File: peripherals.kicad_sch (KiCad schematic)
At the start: 65 parts, among them J401 JTAG, J402 USB_B_Micro, J403 Conn_02x20, J404 Micro_SD_Card_Det2, J405 USB1, J406 USB2, U401 FT230XQ, U403 MX25L1606, U404 TPD4E02B04DQA, U405 AP3417C, U406 AP3417C, U407 AP3417C, X401 XO32

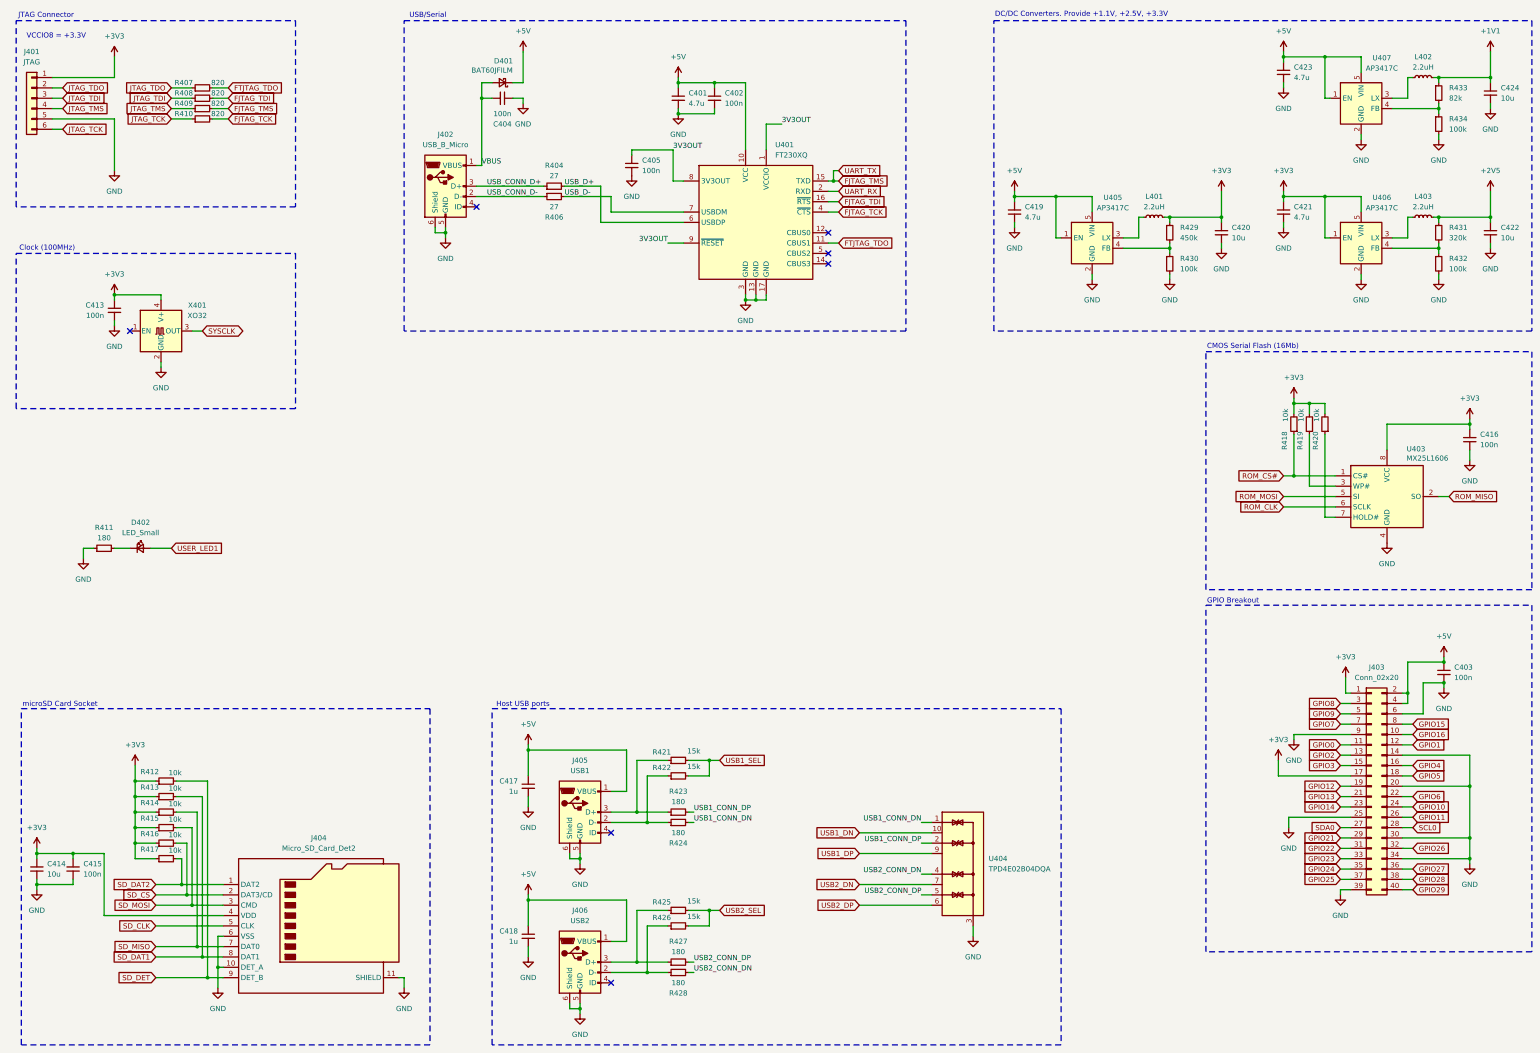
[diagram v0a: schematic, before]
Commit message: First whole routing
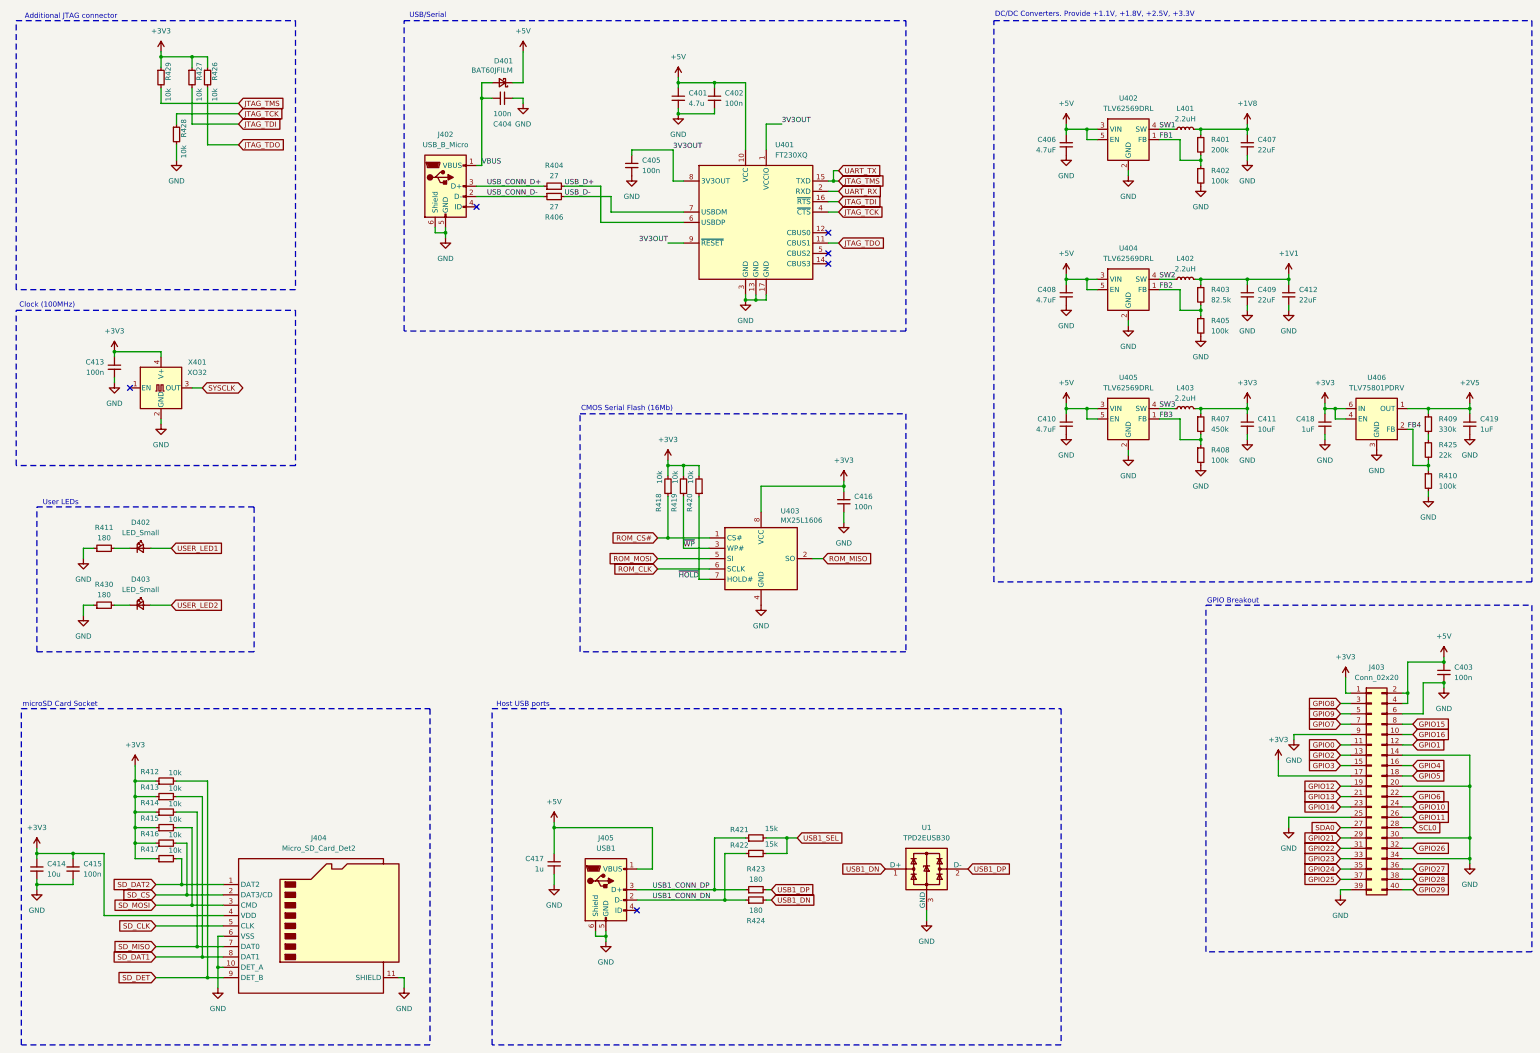
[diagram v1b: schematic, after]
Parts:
- removed C420, C422, C424: 10u, Capacitor_SMD:C_0603_1608Metric, symbol Device:C_Small
- removed C421, C423: 4.7u, Capacitor_SMD:C_0603_1608Metric, symbol Device:C_Small
- removed J401: JTAG, Connector_PinHeader_2.00mm:PinHeader_1x06_P2.00mm_Vertical, symbol Connector_Generic:Conn_01x06
- removed J406: USB2, Connector_USB:USB_Micro-B_Amphenol_10118193-0001LF_Horizontal, symbol Connector:USB_B_Micro
- removed R431: 320k, Resistor_SMD:R_0402_1005Metric, symbol Device:R_Small
- removed R432, R434: 100k, Resistor_SMD:R_0402_1005Metric, symbol Device:R_Small
- removed R433: 82k, Resistor_SMD:R_0402_1005Metric, symbol Device:R_Small
- removed U404: TPD4E02B04DQA, Package_SON:USON-10_2.5x1.0mm_P0.5mm, symbol Power_Protection:TPD4E02B04DQA
- removed U405, U406, U407: AP3417C, Package_TO_SOT_SMD:SOT-23-5, symbol Regulator_Switching_Extra:AP3417C
- added C406, C408, C410: 4.7uF, Capacitor_SMD:C_0603_1608Metric, symbol Device:C_Small
- added C407, C409, C412: 22uF, Capacitor_SMD:C_0603_1608Metric, symbol Device:C_Small
- added C411: 10uF, Capacitor_SMD:C_0603_1608Metric, symbol Device:C_Small
- added D403: LED_Small, LED_SMD:LED_0603_1608Metric, symbol Device:LED_Small
- added R401: 200k, Resistor_SMD:R_0402_1005Metric, symbol Device:R_Small
- added R402, R405: 100k, Resistor_SMD:R_0402_1005Metric, symbol Device:R_Small
- added R403: 82.5k, Resistor_SMD:R_0402_1005Metric, symbol Device:R_Small
- added U1: TPD2EUSB30, Package_TO_SOT_SMD:Texas_DRT-3, symbol Power_Protection:TPD2EUSB30
- added U402, U404, U405: TLV62569DRL, Package_TO_SOT_SMD:SOT-563, symbol Regulator_Switching:TLV62569DRL
- added U406: TLV75801PDRV, Package_SON:WSON-6-1EP_2x2mm_P0.65mm_EP1x1.6mm, symbol Regulator_Linear:TLV75801PDRV
- C403: footprint Capacitor_SMD:C_0201_0603Metric -> Capacitor_SMD:C_0603_1608Metric; MPN (none) -> C14663
- C404, C413: MPN (none) -> C1525
- C417: footprint Capacitor_SMD:C_0402_1005Metric -> Capacitor_SMD:C_0603_1608Metric
- C418: value 1u -> 1uF; MPN (none) -> C52923
- C419: value 4.7u -> 1uF; footprint Capacitor_SMD:C_0603_1608Metric -> Capacitor_SMD:C_0402_1005Metric; MPN (none) -> C52923
- D401: MFN C133103 -> (none); MPN (none) -> C133103
- D402: MPN (none) -> C2286
- J402, J405: MFN C132562 -> (none); MPN (none) -> C132562
- J404: MFN C585350 -> (none); MPN (none) -> C585350
- L401, L402, L403: footprint Inductor_SMD:L_0603_1608Metric -> Inductor_SMD:L_0805_2012Metric; MFN C365953 -> (none); MPN (none) -> C383369
- R407: value 820 -> 450k; MPN (none) -> C5159688
- R408, R410: value 820 -> 100k; MPN (none) -> C25741
- R409: value 820 -> 330k; footprint Resistor_SMD:R_0402_1005Metric -> Resistor_SMD:R_0603_1608Metric; MPN (none) -> C23137
- R412, R413, R414, R415, R416, R417, R418, R419, R420: MPN (none) -> C25744
- R421, R422: MPN (none) -> C25756
- R425: value 15k -> 22k; MPN (none) -> C25768
- R426: value 15k -> 10k; MPN (none) -> C25744
- R427, R428: value 180 -> 10k; MPN (none) -> C25744
- R429: value 450k -> 10k; MPN (none) -> C25744
- R430: value 100k -> 180
- U401: MFN C128629 -> (none); MPN (none) -> C128629
- U403: footprint Package_SON:WSON-8-1EP_6x5mm_P1.27mm_EP3.4x4mm -> Package_SO_Extra:SOP-8-1EP_3.9x4.9mm_P1.27m_EP4.1x3.5mm; MPN (none) -> C3014050
- X401: MFN C4353707 -> (none); MPN (none) -> C4353707
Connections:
- net USB2_CONN_DN is gone; now on net GND: R428.2
- net USB2_CONN_DP is gone; now on net JTAG_TDI: R427.2
- net +1V1: now also C409.1, C412.1, R403.1
- net +2V5: now also C419.1, R409.1, U406.1 (OUT); no longer L403.2
- net +3V3: now also C418.1, L403.2, R407.1, R426.1, R427.1, C411.1, U406.4 (EN), U406.6 (IN); no longer L401.2
- net +5V: now also C406.1, C408.1, C410.1, U402.3 (VIN), U402.5 (EN), U404.3 (VIN), U404.5 (EN), U405.3 (VIN), U405.5 (EN); no longer C418.1, C419.1
- net GND: now also R408.2, R410.2, R430.1, C406.2, C407.2, C408.2, C409.2, C410.2, C411.2, C412.2, R402.2, R405.2, U1.3 (GND), U402.2 (GND), U404.2 (GND), U405.2 (GND), U406.3 (GND), U406.7 (GND); no longer R430.2
- net JTAG_TCK: now also R428.1, U401.4 (~{CTS}); no longer R410.1
- net JTAG_TDI: now also U401.16 (~{RTS}); no longer R408.1
- net JTAG_TDO: now also R426.2, U401.11 (CBUS1); no longer R407.1
- net JTAG_TMS: now also R429.2, U401.15 (TXD); no longer R409.1
- net USB1_CONN_DN: now also J405.2 (D-), R422.1, R424.1; no longer R424.2
- net USB1_CONN_DP: now also J405.3 (D+), R421.1, R423.1; no longer R423.2
- net USB1_DN: now also R424.2, U1.1 (D+)
- net USB1_DP: now also R423.2, U1.2 (D-)
- net at R425.1: now also R409.2; no longer R427.1
- net SW2: now reaches L402.1
- net SW2: now also U404.4 (SW)
- net SW3: now reaches L403.1
- net SW3: now also U405.4 (SW)
- net SW1: now reaches L401.1
- net SW1: now also U402.4 (SW)
- net ~{HOLD}: now reaches R420.1, U403.7 (HOLD#)
- net ~{WP}: now reaches R419.1, U403.3 (WP#)
- removed net FJTAG_TCK: R410.2, U401.4 (~{CTS})
- removed net FJTAG_TDI: R408.2, U401.16 (~{RTS})
- removed net FJTAG_TMS: R409.2, U401.15 (TXD)
- net FTJTAG_TDO renamed FB3
- net FB3: now also R408.1, U405.1 (FB); no longer U401.11 (CBUS1)
- net USB2_SEL renamed FB4
- net FB4: now also R410.1, U406.2 (FB); no longer R426.2
- new net: D403.1 (K), R430.2
- new net +1V8: C407.1, L401.2, R401.1
- new net FB1: R401.2, R402.1, U402.1 (FB)
- new net FB2: R403.2, R405.1, U404.1 (FB)
- new net USER_LED2: D403.2 (A)
- no-connect marks 7 -> 6
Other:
- note added: "Additional JTAG connector"
- note added: "DC/DC Converters. Provide +1.1V, +1.8V, +2.5V, +3.3V"
- note added: "User LEDs"
- note removed: "DC/DC Converters. Provide +1.1V, +2.5V, +3.3V"
- note removed: "JTAG Connector"
- note removed: "VCCIO8 = +3.3V"
- moved on the sheet: C413, C416, C417, J405, R418, R419, R420, R421, R422, R423, R424, U403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
